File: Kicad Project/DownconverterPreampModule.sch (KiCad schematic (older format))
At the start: 17 parts, among them J1 JACK_TRS_6PINS, U1 GALI-1+, U2 MCA1-85L+, U4 LMV751

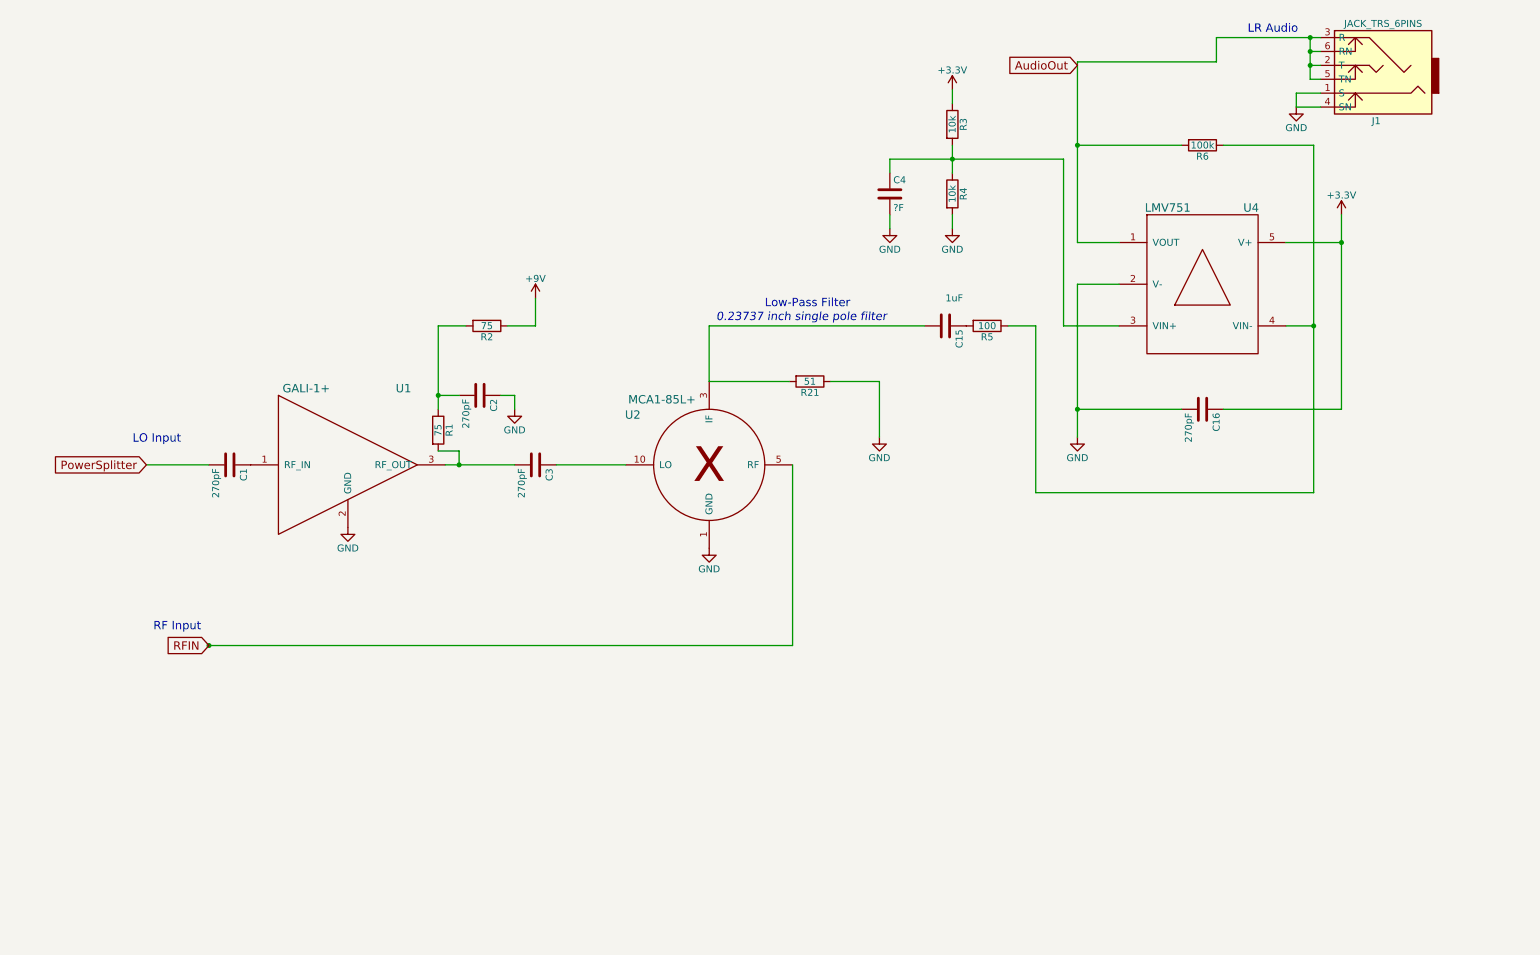
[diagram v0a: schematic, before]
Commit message: Rev 2?
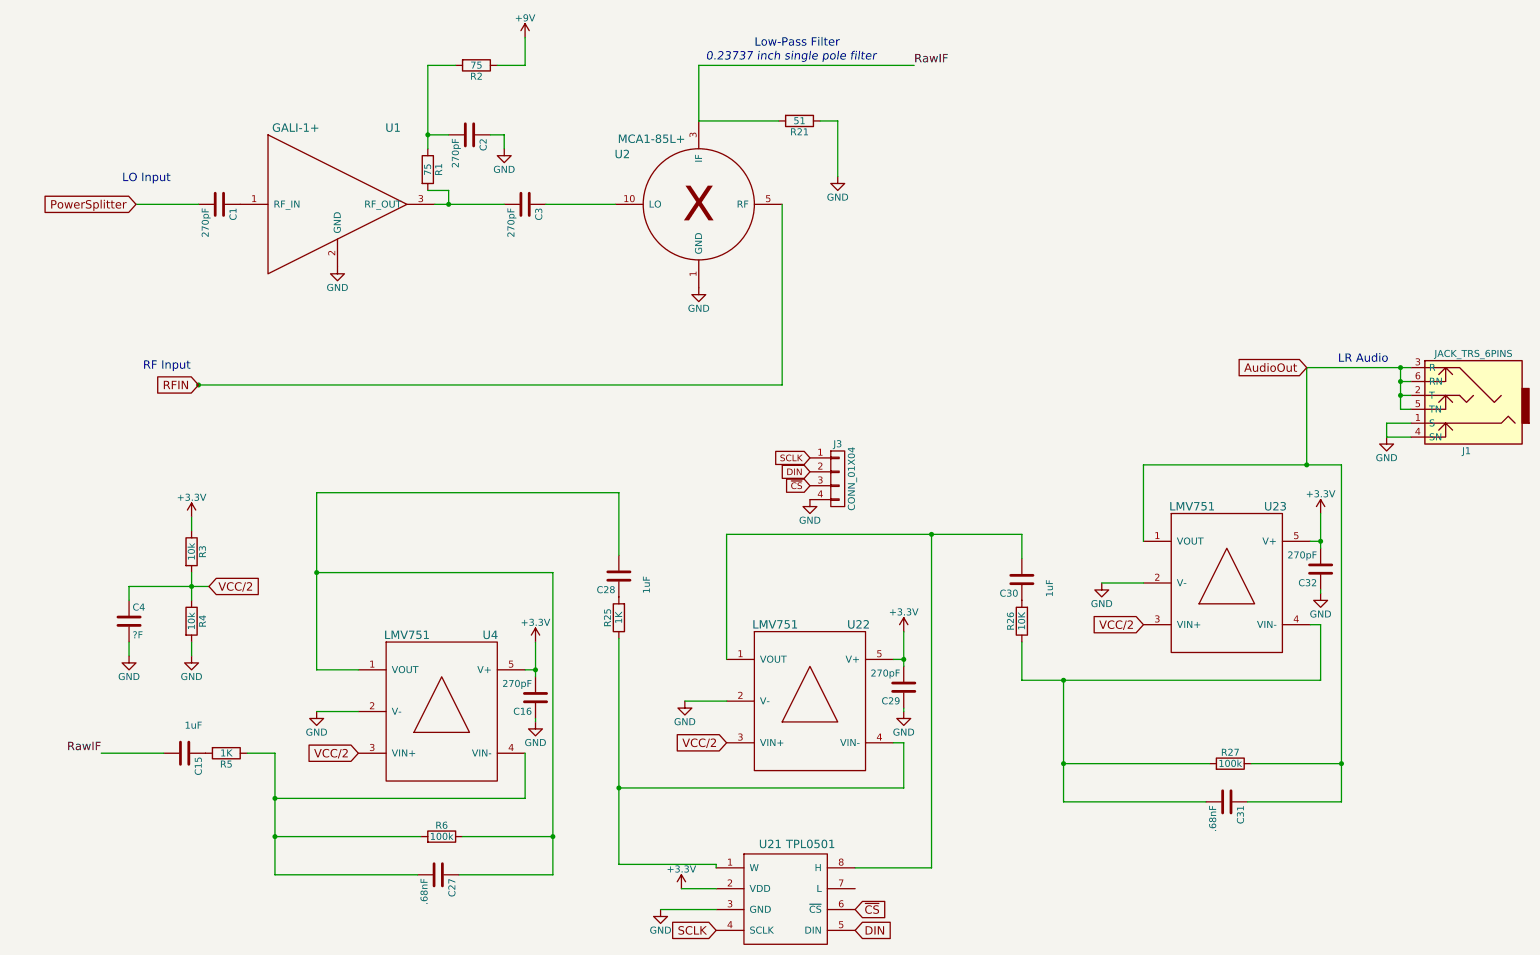
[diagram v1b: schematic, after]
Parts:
- added C27, C31: .68nF, Capacitors_SMD:C_0603, symbol C
- added C28, C30: 1uF, Capacitors_SMD:C_0603, symbol C
- added C29, C32: 270pF, Capacitors_SMD:C_0603, symbol C
- added J3: CONN_01X04, symbol CONN_01X04
- added R25: 1K, Resistors_SMD:R_0603, symbol R
- added R26: 10K, Resistors_SMD:R_0603, symbol R
- added R27: 100k, Resistors_SMD:R_0603, symbol R
- added U21: TPL0501, symbol TPL0501
- added U22, U23: LMV751, RadarComponents:SOT23-5, symbol LMV751
- R5: value 100 -> 1K
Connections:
- net +3V3: now also C16.2, C29.2, C32.2, U21.2 (VDD), U22.5 (V+), U23.5 (V+); no longer C16.1
- net AudioOut: now also C31.1, R27.1, U23.1 (VOUT); no longer R6.2, U4.1 (VOUT)
- net GND: now also C16.1, C29.1, C32.1, J3.4 (P4), U21.3 (GND), U22.2 (V-), U23.2 (V-); no longer C16.2
- net RawIF: now reaches C15.2, R21.2, U2.3 (IF)
- net VCC/2: now reaches C4.1, R3.2, R4.1, U4.3 (VIN+)
- net VCC/2: now also U22.3 (VIN+), U23.3 (VIN+)
- net at R5.1, U4.4 (VIN-): now also R6.2, C27.2; no longer R6.1
- new net: C27.1, C28.2, R6.1, U4.1 (VOUT)
- new net: C30.2, U21.8 (H), U22.1 (VOUT)
- new net: R25.1, U21.1 (W), U22.4 (VIN-)
- new net: C31.2, R26.1, R27.2, U23.4 (VIN-)
- new net: C28.1, R25.2
- new net: C30.1, R26.2
- new net DIN: J3.2 (P2), U21.5 (DIN)
- new net SCLK: J3.1 (P1), U21.4 (SCLK)
- new net ~CS: J3.3 (P3), U21.6 (~CS)
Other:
- moved on the sheet: C1, C15, C16, C2, C3, C4, J1, R1, R2, R21, R3, R4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
